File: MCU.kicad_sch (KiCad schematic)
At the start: 19 parts, among them U1 NRF52810-QCAA-E-R7, Y1 32.768kHz, Y2 32MHz

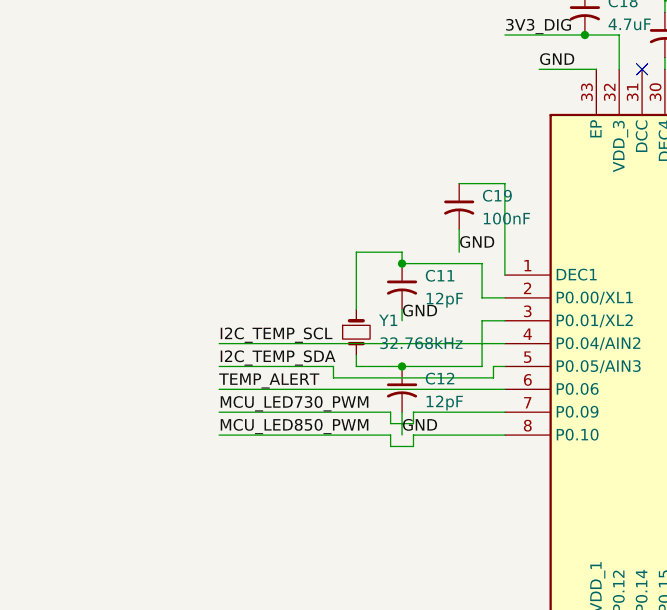
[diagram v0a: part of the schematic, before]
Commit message: footprint
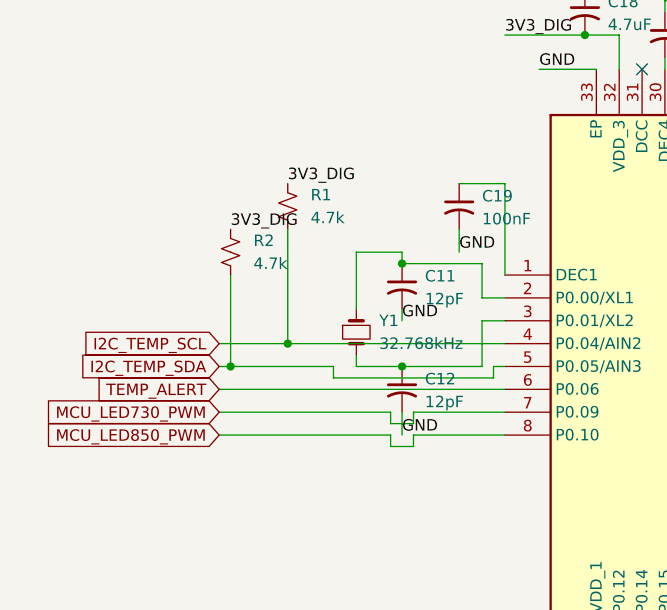
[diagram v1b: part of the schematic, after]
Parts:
- added R1, R2: 4.7k, symbol Device:R_Small_US
- U1: footprint QFN50P500X500X90-33N -> NRF52810-QCAA-E-R7:QFN50P500X500X90-33N
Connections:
- net 3V3_DIG: now also R1.1, R2.1
- net I2C_TEMP_SCL: now also R1.2
- net I2C_TEMP_SDA: now also R2.2
